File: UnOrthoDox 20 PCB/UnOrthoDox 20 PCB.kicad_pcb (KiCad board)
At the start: 2 copper layers, 76.2 x 94.2 mm, 81 parts, among them J1 Conn_01x02, SW1 SW_MX_HotSwap, SW10 SW_MX_HotSwap, SW11 SW_MX_HotSwap, SW12 SW_MX_HotSwap, SW13 SW_MX_HotSwap, SW14 SW_MX_HotSwap, SW15 SW_MX_HotSwap, SW16 SW_MX_HotSwap, SW16A1 SW_MX_HotSwap, SW17 SW_MX_HotSwap, SW17A1 SW_MX_HotSwap, SW18 SW_MX_HotSwap, SW19 SW_MX_HotSwap, SW2 SW_MX_HotSwap, SW20 SW_MX_HotSwap, SW3 SW_MX_HotSwap, SW4 SW_MX_HotSwap, SW5 SW_MX_HotSwap, SW6 SW_MX_HotSwap, SW7 SW_MX_HotSwap, SW8 SW_MX_HotSwap, SW8A1 SW_MX_HotSwap, SW9 SW_MX_HotSwap, U1 ProMicro

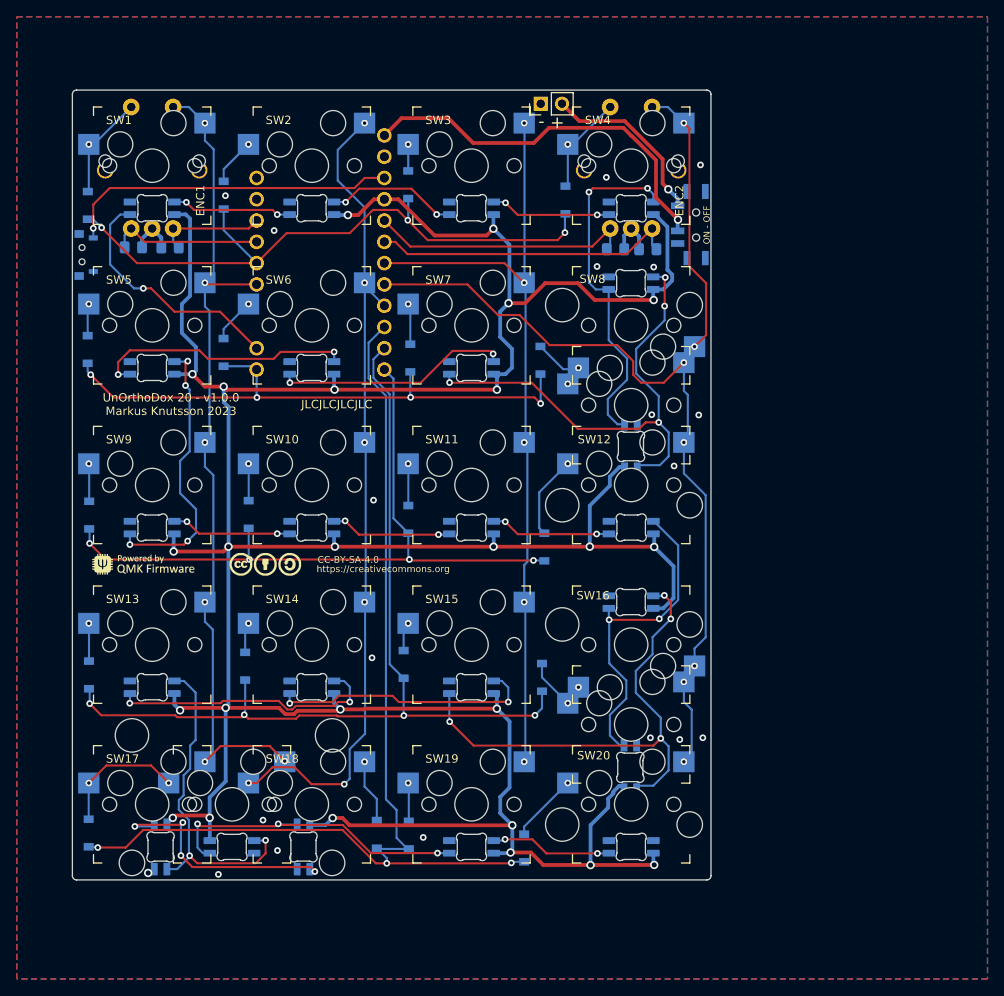
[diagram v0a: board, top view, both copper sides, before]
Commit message: Added 17
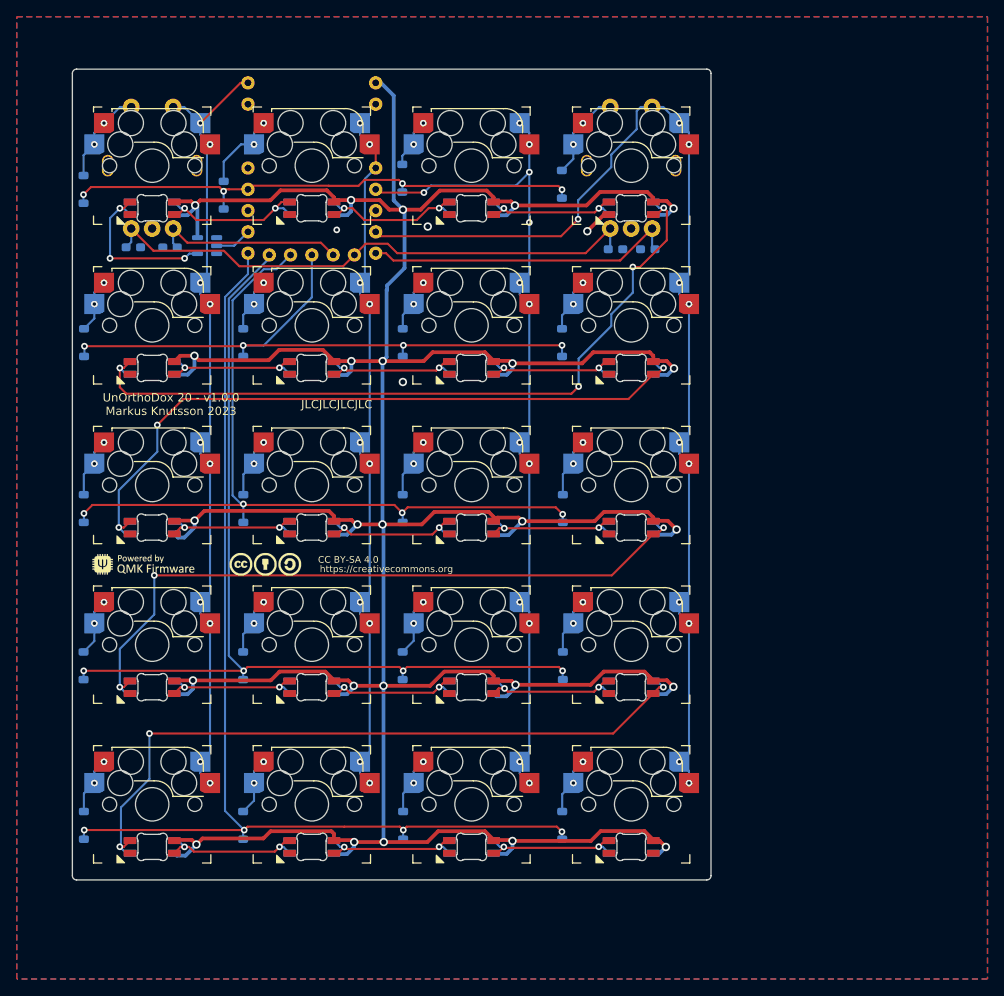
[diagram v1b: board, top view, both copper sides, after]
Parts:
- removed J1: Conn_01x02, Connector_PinHeader_2.54mm:PinHeader_1x02_P2.54mm_Vertical
- removed LED16A1, LED17A1, LED8A1: SK6812, Keyboard RGB:RGB_SK6812MINI-E
- removed RES1: TS-A002, Keyboard Common:YTS-A002
- removed ST1, ST2, ST3: Stabilizer_2u_MX, Keyboard Stabilizer:Stabilizer_Cherry_MX_2.00u
- removed SW16A1, SW17A1, SW8A1: SW_MX_HotSwap, Keyboard Switches:SW_MX_HotSwap
- removed SW_SLIDE_1: MSK12C02, Keyboard Common:MSK12C02
- added RZ1: RP2040-Zero, Keyboard Controllers:RP2040-Zero_reverse_mount_flipped, B.Cu at (147.8, 54.7)
- C1, C2, C3, C4: value 100nF -> C_Small; footprint Capacitor_SMD:C_0805_2012Metric_Pad1.18x1.45mm_HandSolder -> Capacitor_SMD:C_0603_1608Metric_Pad1.08x0.95mm_HandSolder
- ENC1, ENC2: footprint Keyboard Encoders:Encoder_Alps_EC11E_Offset_pad -> Keyboard Encoders:Encoder_Alps_EC11E_Small
- RGB1: renamed from LED1; value SK6812 -> SK6812MINI-E; footprint Keyboard RGB:RGB_SK6812MINI-E -> Keyboard RGB:MX_SK6812MINI-E_REVERSIBLE
- RGB10: renamed from LED10; value SK6812 -> SK6812MINI-E; footprint Keyboard RGB:RGB_SK6812MINI-E -> Keyboard RGB:MX_SK6812MINI-E_REVERSIBLE
- RGB11: renamed from LED11; value SK6812 -> SK6812MINI-E; footprint Keyboard RGB:RGB_SK6812MINI-E -> Keyboard RGB:MX_SK6812MINI-E_REVERSIBLE
- RGB12: renamed from LED12; value SK6812 -> SK6812MINI-E; footprint Keyboard RGB:RGB_SK6812MINI-E -> Keyboard RGB:MX_SK6812MINI-E_REVERSIBLE
- RGB13: renamed from LED13; value SK6812 -> SK6812MINI-E; footprint Keyboard RGB:RGB_SK6812MINI-E -> Keyboard RGB:MX_SK6812MINI-E_REVERSIBLE
- RGB14: renamed from LED14; value SK6812 -> SK6812MINI-E; footprint Keyboard RGB:RGB_SK6812MINI-E -> Keyboard RGB:MX_SK6812MINI-E_REVERSIBLE
- RGB15: renamed from LED15; value SK6812 -> SK6812MINI-E; footprint Keyboard RGB:RGB_SK6812MINI-E -> Keyboard RGB:MX_SK6812MINI-E_REVERSIBLE
- RGB16: renamed from LED16; value SK6812 -> SK6812MINI-E; footprint Keyboard RGB:RGB_SK6812MINI-E -> Keyboard RGB:MX_SK6812MINI-E_REVERSIBLE
- RGB17: renamed from LED17; value SK6812 -> SK6812MINI-E; footprint Keyboard RGB:RGB_SK6812MINI-E -> Keyboard RGB:MX_SK6812MINI-E_REVERSIBLE
- RGB18: renamed from LED18; value SK6812 -> SK6812MINI-E; footprint Keyboard RGB:RGB_SK6812MINI-E -> Keyboard RGB:MX_SK6812MINI-E_REVERSIBLE
- RGB19: renamed from LED19; value SK6812 -> SK6812MINI-E; footprint Keyboard RGB:RGB_SK6812MINI-E -> Keyboard RGB:MX_SK6812MINI-E_REVERSIBLE
- RGB2: renamed from LED2; value SK6812 -> SK6812MINI-E; footprint Keyboard RGB:RGB_SK6812MINI-E -> Keyboard RGB:MX_SK6812MINI-E_REVERSIBLE
- RGB20: renamed from LED20; value SK6812 -> SK6812MINI-E; footprint Keyboard RGB:RGB_SK6812MINI-E -> Keyboard RGB:MX_SK6812MINI-E_REVERSIBLE
- RGB3: renamed from LED3; value SK6812 -> SK6812MINI-E; footprint Keyboard RGB:RGB_SK6812MINI-E -> Keyboard RGB:MX_SK6812MINI-E_REVERSIBLE
- RGB4: renamed from LED4; value SK6812 -> SK6812MINI-E; footprint Keyboard RGB:RGB_SK6812MINI-E -> Keyboard RGB:MX_SK6812MINI-E_REVERSIBLE
- RGB5: renamed from LED5; value SK6812 -> SK6812MINI-E; footprint Keyboard RGB:RGB_SK6812MINI-E -> Keyboard RGB:MX_SK6812MINI-E_REVERSIBLE
- RGB6: renamed from LED6; value SK6812 -> SK6812MINI-E; footprint Keyboard RGB:RGB_SK6812MINI-E -> Keyboard RGB:MX_SK6812MINI-E_REVERSIBLE
- RGB7: renamed from LED7; value SK6812 -> SK6812MINI-E; footprint Keyboard RGB:RGB_SK6812MINI-E -> Keyboard RGB:MX_SK6812MINI-E_REVERSIBLE
- RGB8: renamed from LED8; value SK6812 -> SK6812MINI-E; footprint Keyboard RGB:RGB_SK6812MINI-E -> Keyboard RGB:MX_SK6812MINI-E_REVERSIBLE
- RGB9: renamed from LED9; value SK6812 -> SK6812MINI-E; footprint Keyboard RGB:RGB_SK6812MINI-E -> Keyboard RGB:MX_SK6812MINI-E_REVERSIBLE
- SW1, SW10, SW11, SW12, SW13, SW14, SW15, SW16, SW17, SW18, SW19, SW2, SW20, SW3, SW4, SW5, SW6, SW7, SW8, SW9: footprint Keyboard Switches:SW_MX_HotSwap -> Keyboard Switches:SW_MX_HotSwap_Reversible
- U1: value ProMicro -> SN74LV1T34DBV; footprint Keyboard Controllers:ArduinoProMicro-BackSide_special -> Package_TO_SOT_SMD:SOT-23-5; moved to B.Cu
- moved D18 16.0 mm to (130.6, 121.4)
- moved RGB16 15.2 mm to (176.9, 104.9), turned to 180 degrees
- moved RGB8 15.2 mm to (176.9, 66.8), turned to 180 degrees
- moved U1 13.6 mm to (126.3, 52.2), turned to 180 degrees
- moved RGB18 6.08 mm to (138.8, 123.9), turned to 180 degrees
- moved D20 5.28 mm to (168.7, 121.4)
- moved D12 5.10 mm to (168.8, 83.6)
- moved RGB1 5.08 mm to (119.8, 47.7), turned to 180 degrees
- moved RGB2 5.08 mm to (138.8, 47.7), turned to 180 degrees
- moved RGB3 5.08 mm to (157.9, 47.7), turned to 180 degrees
- moved RGB4 5.08 mm to (176.9, 47.7), turned to 180 degrees
- moved RGB5 5.08 mm to (119.8, 66.8), turned to 180 degrees
- moved RGB6 5.08 mm to (138.8, 66.8), turned to 180 degrees
- moved RGB7 5.08 mm to (157.9, 66.8), turned to 180 degrees
- moved RGB10 5.08 mm to (138.8, 85.8), turned to 180 degrees
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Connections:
- net C renamed Net-(D17-A)
- net ENC1 renamed EncA
- net ENC2 renamed EncB
- C1 pad 1: Enc1A -> Enc_1
- C2 pad 2: Enc1B -> Enc_2
- C3 pad 1: Enc2A -> Enc_1
- C4 pad 2: Enc2B -> Enc_3
- D16 pad 2: B -> Net-(D16-A)
- D18 pad 2: Net-(D18-Pad2) -> Net-(D18-A)
- D8 pad 2: A -> Net-(D8-A)
- ENC1 pad A: Enc1A -> Enc_1
- ENC1 pad B: Enc1B -> Enc_2
- ENC2 pad A: Enc2A -> Enc_1
- ENC2 pad B: Enc2B -> Enc_3
- RGB1 pad 1: GND -> +5V
- RGB1 pad 2: RGB -> Net-(RGB1-DOUT)
- RGB1 pad 3: VCC -> GND
- RGB1 pad 4: Net-(LED1-Pad4) -> RGB_5
- RGB10 pad 1: GND -> +5V
- RGB10 pad 2: Net-(LED10-Pad2) -> Net-(RGB10-DOUT)
- RGB10 pad 3: VCC -> GND
- RGB10 pad 4: Net-(LED10-Pad4) -> Net-(RGB10-DIN)
- RGB11 pad 1: GND -> +5V
- RGB11 pad 2: Net-(LED10-Pad4) -> Net-(RGB11-DOUT)
- RGB11 pad 3: VCC -> GND
- RGB11 pad 4: Net-(LED11-Pad4) -> Net-(RGB10-DOUT)
- RGB12 pad 1: GND -> +5V
- RGB12 pad 2: Net-(LED11-Pad4) -> Net-(RGB12-DOUT)
- RGB12 pad 3: VCC -> GND
- RGB12 pad 4: Net-(LED12-Pad4) -> Net-(RGB11-DOUT)
- RGB13 pad 1: GND -> +5V
- RGB13 pad 3: VCC -> GND
- RGB13 pad 4: Net-(LED13-Pad4) -> Net-(RGB12-DOUT)
- RGB14 pad 1: GND -> +5V
- RGB14 pad 3: VCC -> GND
- RGB15 pad 1: GND -> +5V
- RGB15 pad 3: VCC -> GND
- RGB16 pad 1: GND -> +5V
- RGB16 pad 2: Net-(LED12-Pad4) -> Net-(RGB16-DOUT)
- RGB16 pad 3: VCC -> GND
- RGB17 pad 1: GND -> +5V
- RGB17 pad 2: Net-(LED13-Pad4) -> Net-(RGB17-DOUT)
- RGB17 pad 3: VCC -> GND
- RGB17 pad 4: Net-(LED17-Pad4) -> Net-(RGB16-DOUT)
- RGB18 pad 1: GND -> +5V
- RGB18 pad 2: Net-(LED17-Pad4) -> Net-(RGB18-DOUT)
- RGB18 pad 3: VCC -> GND
- RGB18 pad 4: Net-(LED17A1-Pad4) -> Net-(RGB17-DOUT)
- RGB19 pad 1: GND -> +5V
- RGB19 pad 2: Net-(LED17A1-Pad4) -> Net-(RGB19-DOUT)
- RGB19 pad 3: VCC -> GND
- RGB19 pad 4: Net-(LED19-Pad4) -> Net-(RGB18-DOUT)
- RGB2 pad 1: GND -> +5V
- RGB2 pad 2: Net-(LED1-Pad4) -> Net-(RGB2-DOUT)
- RGB2 pad 3: VCC -> GND
- RGB2 pad 4: Net-(LED2-Pad4) -> Net-(RGB1-DOUT)
- RGB20 pad 1: GND -> +5V
- RGB20 pad 2: Net-(LED19-Pad4) -> unconnected-(RGB20-DOUT-Pad2)
- RGB20 pad 3: VCC -> GND
- RGB20 pad 4: unconnected-(LED20-Pad4) -> Net-(RGB19-DOUT)
- RGB3 pad 1: GND -> +5V
- RGB3 pad 2: Net-(LED2-Pad4) -> Net-(RGB3-DOUT)
- RGB3 pad 3: VCC -> GND
- RGB3 pad 4: Net-(LED3-Pad4) -> Net-(RGB2-DOUT)
- RGB4 pad 1: GND -> +5V
- RGB4 pad 2: Net-(LED3-Pad4) -> Net-(RGB4-DOUT)
- RGB4 pad 3: VCC -> GND
- RGB4 pad 4: Net-(LED4-Pad4) -> Net-(RGB3-DOUT)
- RGB5 pad 1: GND -> +5V
- RGB5 pad 3: VCC -> GND
- RGB5 pad 4: Net-(LED5-Pad4) -> Net-(RGB4-DOUT)
- RGB6 pad 1: GND -> +5V
- RGB6 pad 3: VCC -> GND
- RGB7 pad 1: GND -> +5V
- RGB7 pad 3: VCC -> GND
- RGB8 pad 1: GND -> +5V
- RGB8 pad 2: Net-(LED4-Pad4) -> Net-(RGB8-DOUT)
- RGB8 pad 3: VCC -> GND
- RGB9 pad 1: GND -> +5V
- RGB9 pad 2: Net-(LED5-Pad4) -> Net-(RGB10-DIN)
- RGB9 pad 3: VCC -> GND
- RGB9 pad 4: Net-(LED10-Pad2) -> Net-(RGB8-DOUT)
- SW16 pad 1: Col3 -> Net-(D16-A)
- SW16 pad 2: B -> Col3
- SW18 pad 1: Col1 -> Net-(D18-A)
- SW18 pad 2: Net-(D18-Pad2) -> Col1
- SW8 pad 1: Col3 -> Net-(D8-A)
- SW8 pad 2: A -> Col3
- U1 pad 4: GND -> RGB_5
- U1 pad 5: Enc1B -> +5V
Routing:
- net +5V: track 0.00 -> 485.6 mm, vias 0 -> 25
- net VCC: track 410.0 -> 0.00 mm, vias 25 -> 0
- net Net-(RGB4-DOUT): track 0.00 -> 90.2 mm, vias 0 -> 4
- net Net-(RGB16-DOUT): track 0.00 -> 83.2 mm, vias 0 -> 3
- net Net-(RGB12-DOUT): track 0.00 -> 82.8 mm, vias 0 -> 3
- net Net-(RGB8-DOUT): track 0.00 -> 82.2 mm, vias 0 -> 3
- net Enc_1: track 0.00 -> 66.9 mm
- net /RAW: track 46.4 -> 0.00 mm, vias 1 -> 0
- net Net-(RGB15-DOUT): track 60.2 -> 17.9 mm, vias 4 -> 2
- net Net-(LED4-Pad4): track 41.9 -> 0.00 mm, vias 2 -> 0
- net Net-(RGB7-DOUT): track 58.4 -> 17.7 mm, vias 4 -> 2
- net Net-(LED13-Pad4): track 40.2 -> 0.00 mm, vias 2 -> 0
- net Net-(RES1-Pad1): track 40.0 -> 0.00 mm, vias 1 -> 0
- net Net-(LED12-Pad4): track 38.9 -> 0.00 mm, vias 2 -> 0
- net Net-(LED17A1-Pad4): track 38.6 -> 0.00 mm, vias 3 -> 0
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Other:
- board size 76.2 x 94.2 mm -> 76.2 x 96.7 mm
- board text removed: "- +"
- board text removed: "RESET"
